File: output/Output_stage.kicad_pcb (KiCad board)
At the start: 2 copper layers, 64.8 x 27.9 mm, 12 parts, among them J1 Conn_01x03_Socket, J2 Control/LED, J3 Control/LED, Q1 BTA41, U1 MOC3041M

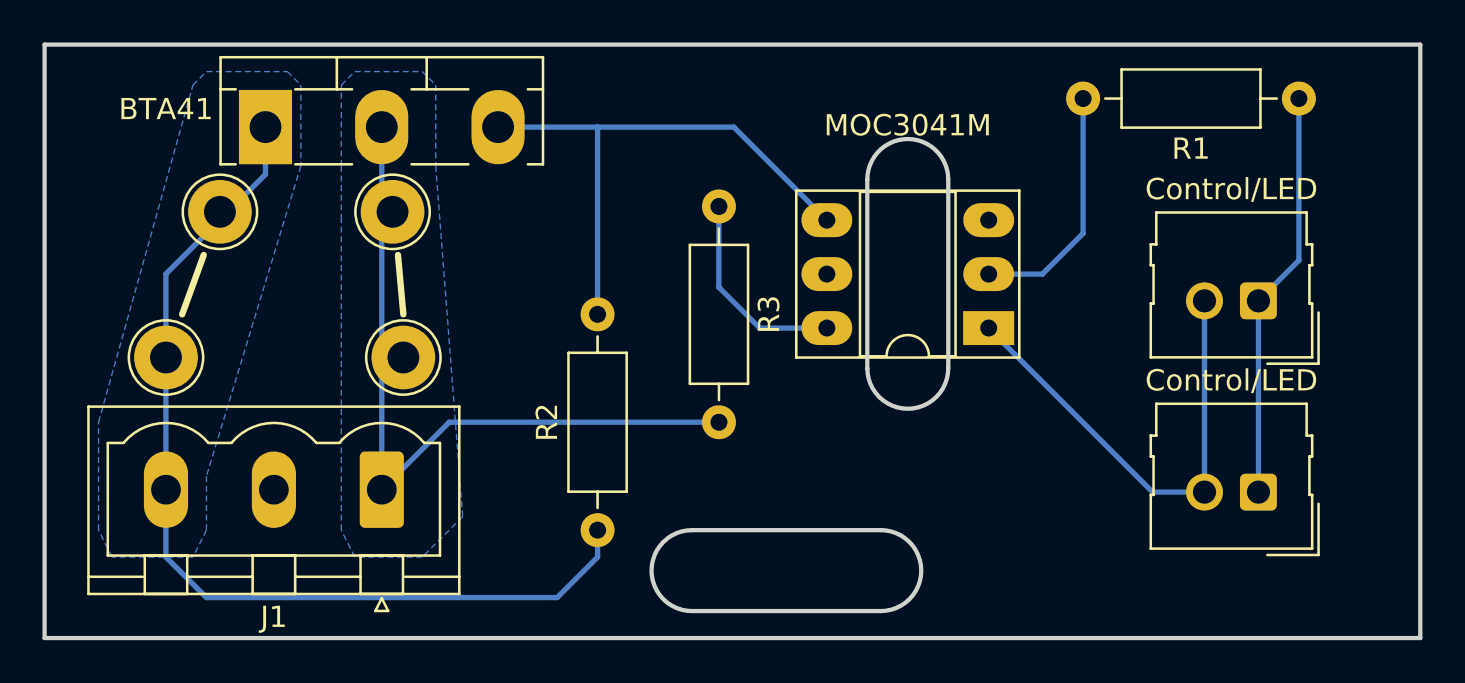
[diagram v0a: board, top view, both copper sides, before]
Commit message: Tuning + labels
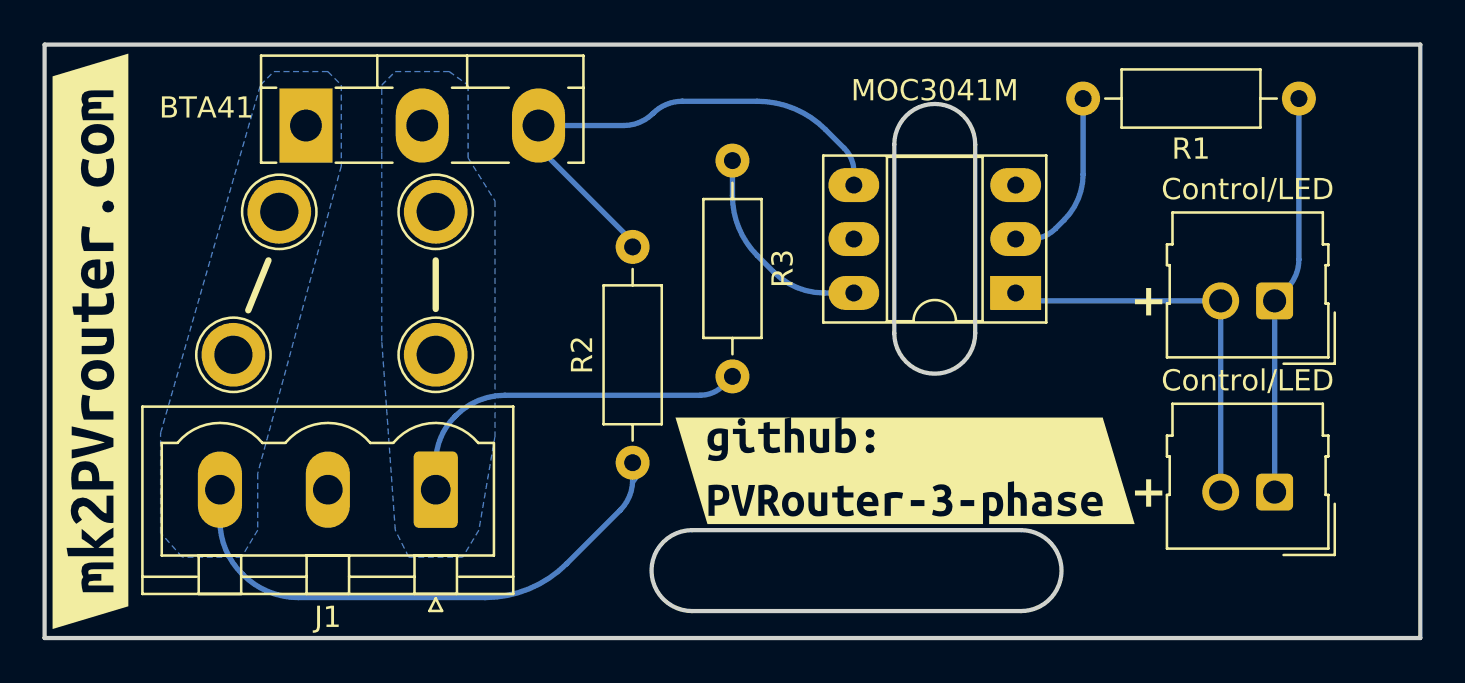
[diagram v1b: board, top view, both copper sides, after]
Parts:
- added kibuzzard-6431D11C: G***, kibuzzard-6431D11C, F.Cu at (39.6, 41.9)
- added kibuzzard-6431D738: G***, kibuzzard-6431D738, F.Cu at (78.0, 48.0)
- moved R2 3.58 mm to (65.2, 47.6)
- moved REF** 3.18 mm to (46.4, 42.5)
- moved REF** 2.79 mm to (48.5, 35.8)
- moved J1 2.54 mm to (55.9, 48.9)
- moved R3 2.25 mm to (69.8, 33.4)
- moved U1 2.08 mm to (83.2, 39.6)
- moved REF** 2.03 mm to (55.9, 35.8)
- moved Q1 1.91 mm to (49.8, 31.8)
- moved REF** 1.53 mm to (55.9, 42.5)
- moved J2 0.76 mm to (95.4, 40.0)
- moved J3 0.76 mm to (95.4, 49.0)
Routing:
- net LINE: track 34.3 -> 17.3 mm
- net S/LINE: track 45.4 -> 29.2 mm
- net Net-(J2-Pin_2): track 22.4 -> 18.0 mm
- net Net-(R1-Pad2): track 11.6 -> 8.51 mm
- net Net-(Q1-G): track 26.1 -> 24.8 mm
- net Net-(J2-Pin_1): track 19.3 -> 18.8 mm
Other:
- outline, holes or cut-outs redrawn
- board text added: "+"
